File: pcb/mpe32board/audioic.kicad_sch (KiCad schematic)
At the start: 13 parts, among them J49 AudioJack3_SwitchT, U1 TAC5212IRGER

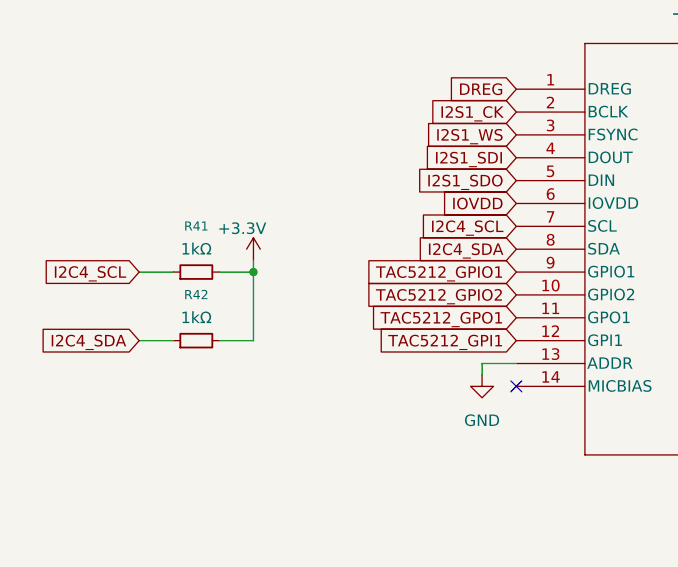
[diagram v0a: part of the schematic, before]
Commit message: routed ram
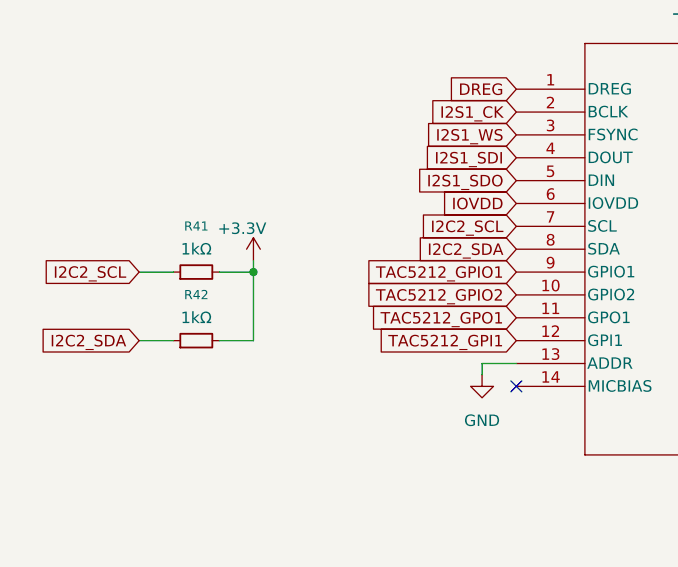
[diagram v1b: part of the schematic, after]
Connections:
- net I2C4_SCL renamed I2C2_SCL
- net I2C4_SDA renamed I2C2_SDA
